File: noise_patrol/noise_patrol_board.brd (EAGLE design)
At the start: 53.3 x 57.1 mm, 13 parts, among them IC1 4511D, Q1 TIP31C, U1 OPA345NA/3K

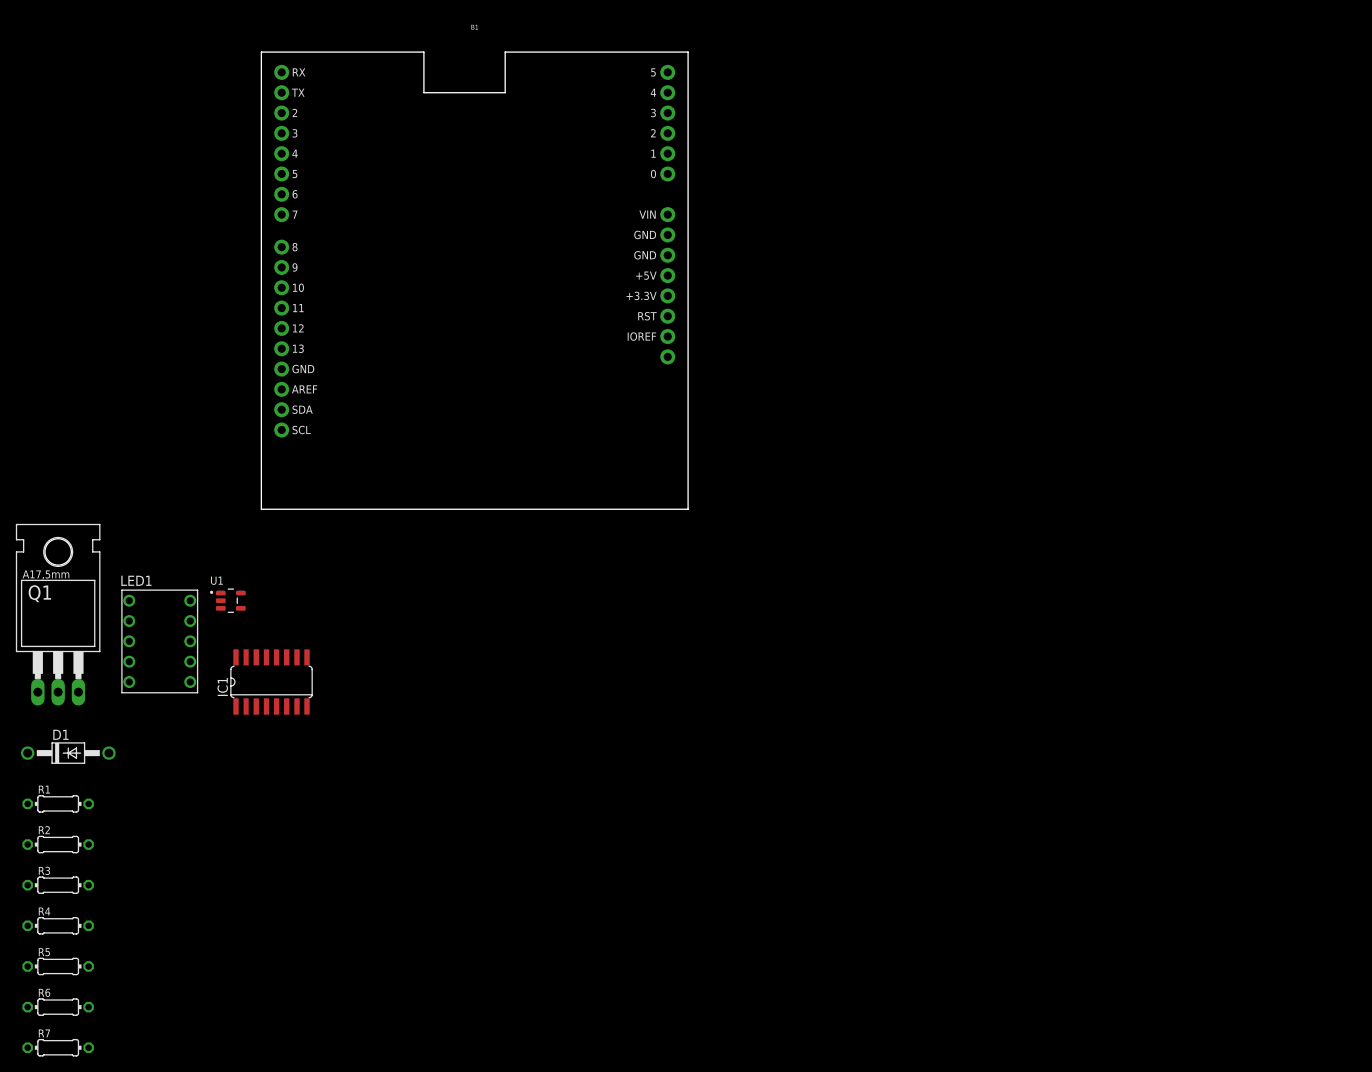
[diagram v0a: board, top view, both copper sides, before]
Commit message: Saving Progress: Added More parts and starting to understand the software
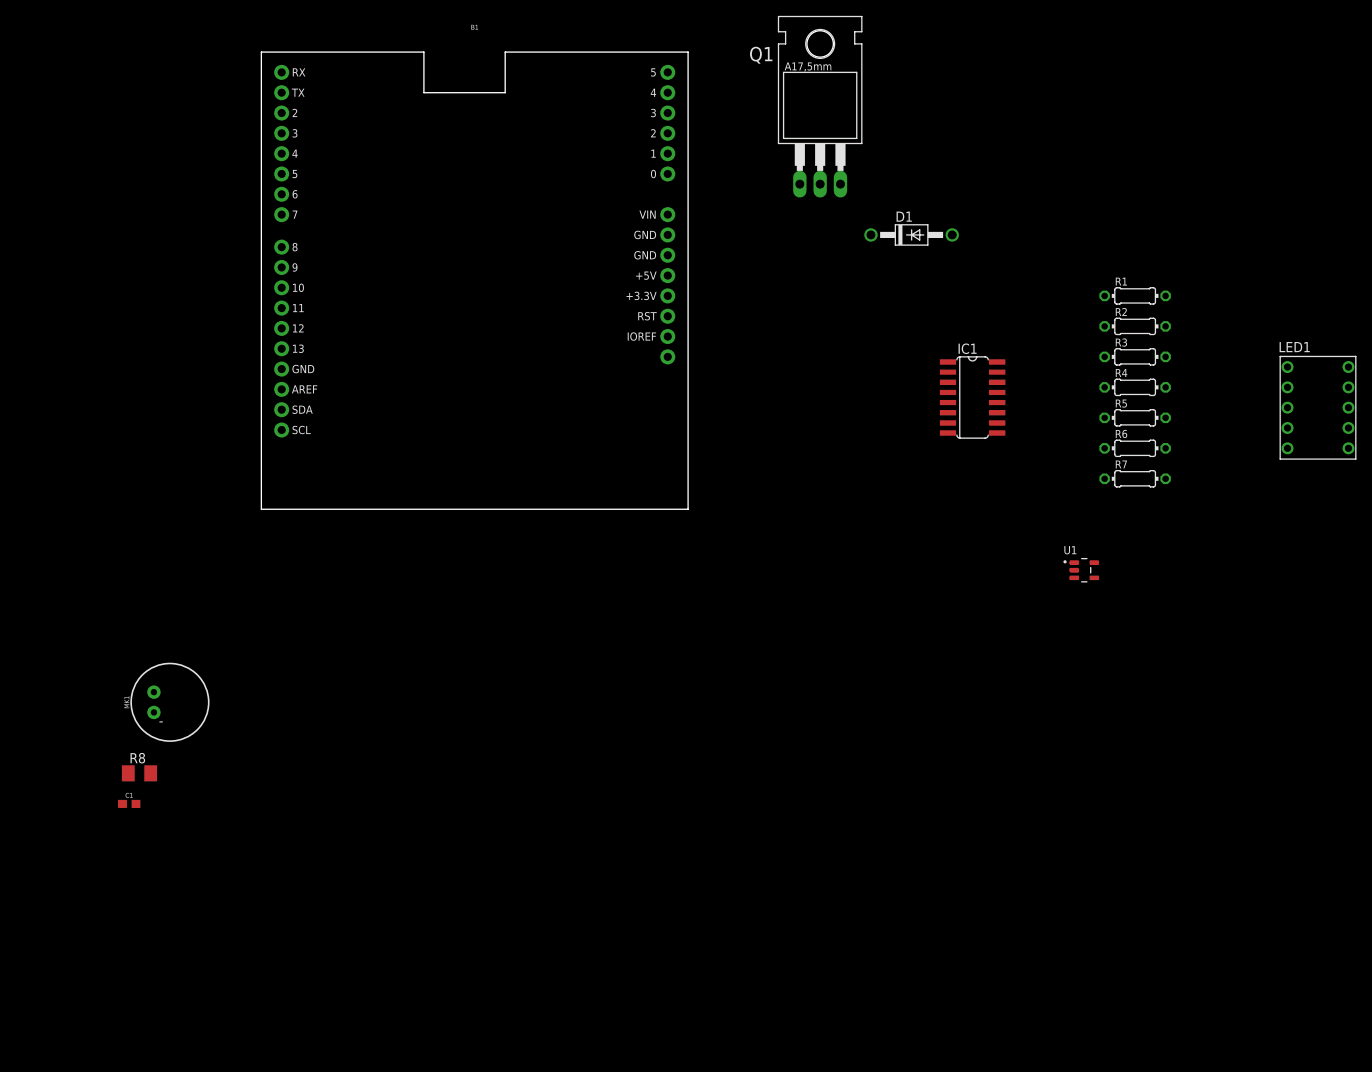
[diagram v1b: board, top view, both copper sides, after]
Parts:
- added C1: 2.2\muF, SparkFun-Capacitors:0603
- added MK1: MIC-PTH, SparkFun-Sensors:MICROPHONE-PTH-9.7MM
- added R8: (no value), rcl:M1206
- R1, R2, R3, R4, R5, R6, R7: value (none) -> 220
- moved R7 152.3 mm to (41.9, 20.3)
- moved R6 151.7 mm to (41.9, 24.1)
- moved R5 151.1 mm to (41.9, 27.9)
- moved R4 150.5 mm to (41.9, 31.8)
- moved R3 149.9 mm to (41.9, 35.6)
- moved R2 149.4 mm to (41.9, 39.4)
- moved R1 148.8 mm to (41.9, 43.2)
- moved LED1 147.7 mm to (64.8, 29.2)
- moved D1 123.7 mm to (14.0, 50.8)
- moved Q1 114.5 mm to (2.54, 63.5)
- moved U1 106.7 mm to (35.6, 8.89)
- moved IC1 94.6 mm to (21.6, 30.5), turned to 270 degrees
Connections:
- net N$1 renamed TOOL
- net V+ renamed +5V
- removed net V-: U1.2
- new net 5V: IC1.3, IC1.4, R8.1
- new net GND: LED1.1, LED1.6, U1.2
- new net N$14: B1.D4, IC1.7
- new net N$15: B1.D5, IC1.1
- new net N$16: B1.D6, IC1.2
- new net N$17: B1.D7, IC1.6
- new net N$18: B1.A0, U1.1
- new net N$19: B1.D8, IC1.5
- new net N$20: C1.1, MK1.OUT, R8.2
